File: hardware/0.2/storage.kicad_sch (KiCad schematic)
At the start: 8 parts, among them J1 Micro_SD_Card, U3 S27KS0641

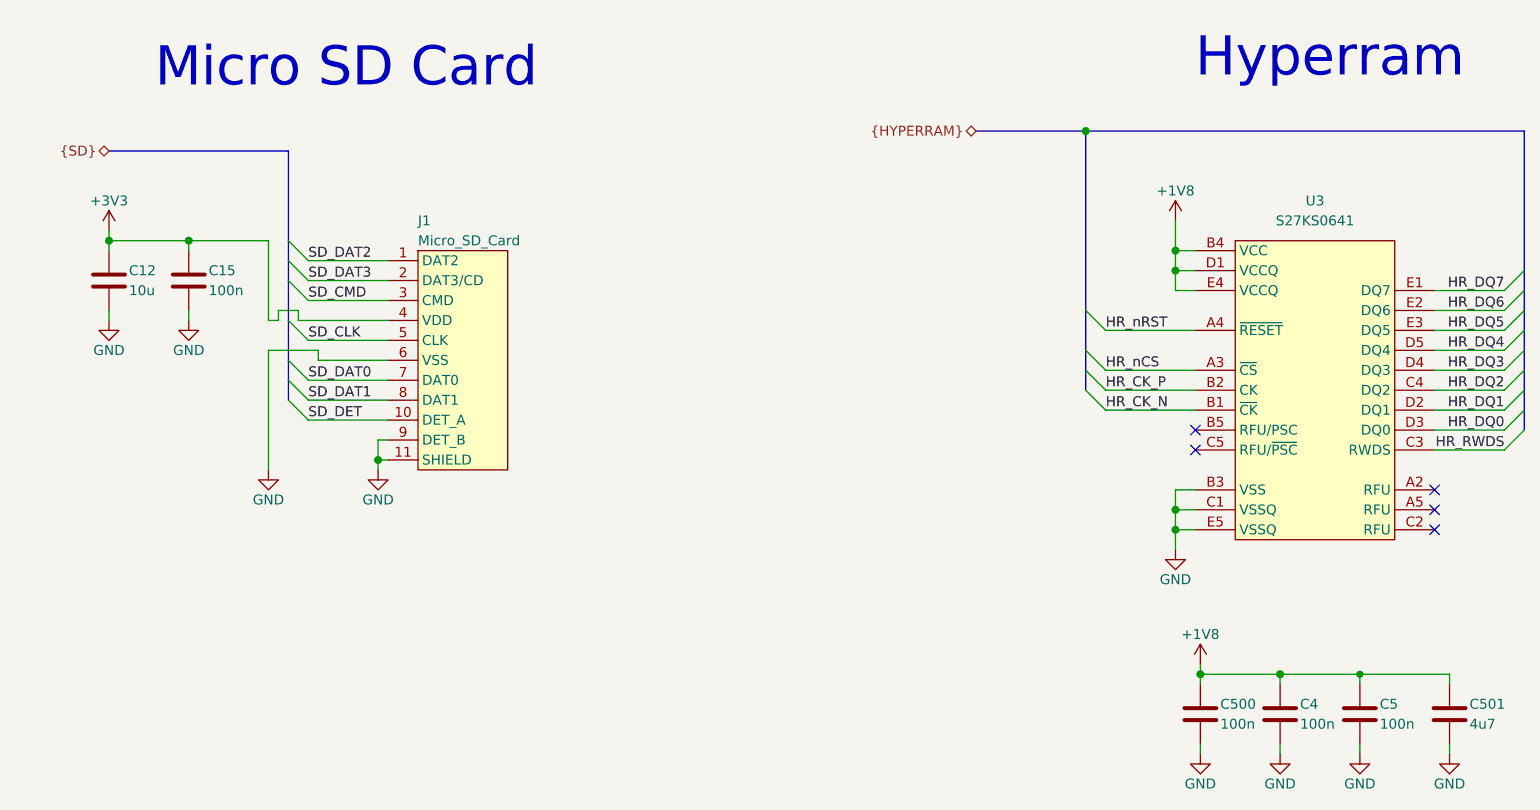
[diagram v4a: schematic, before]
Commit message: nightly version bump
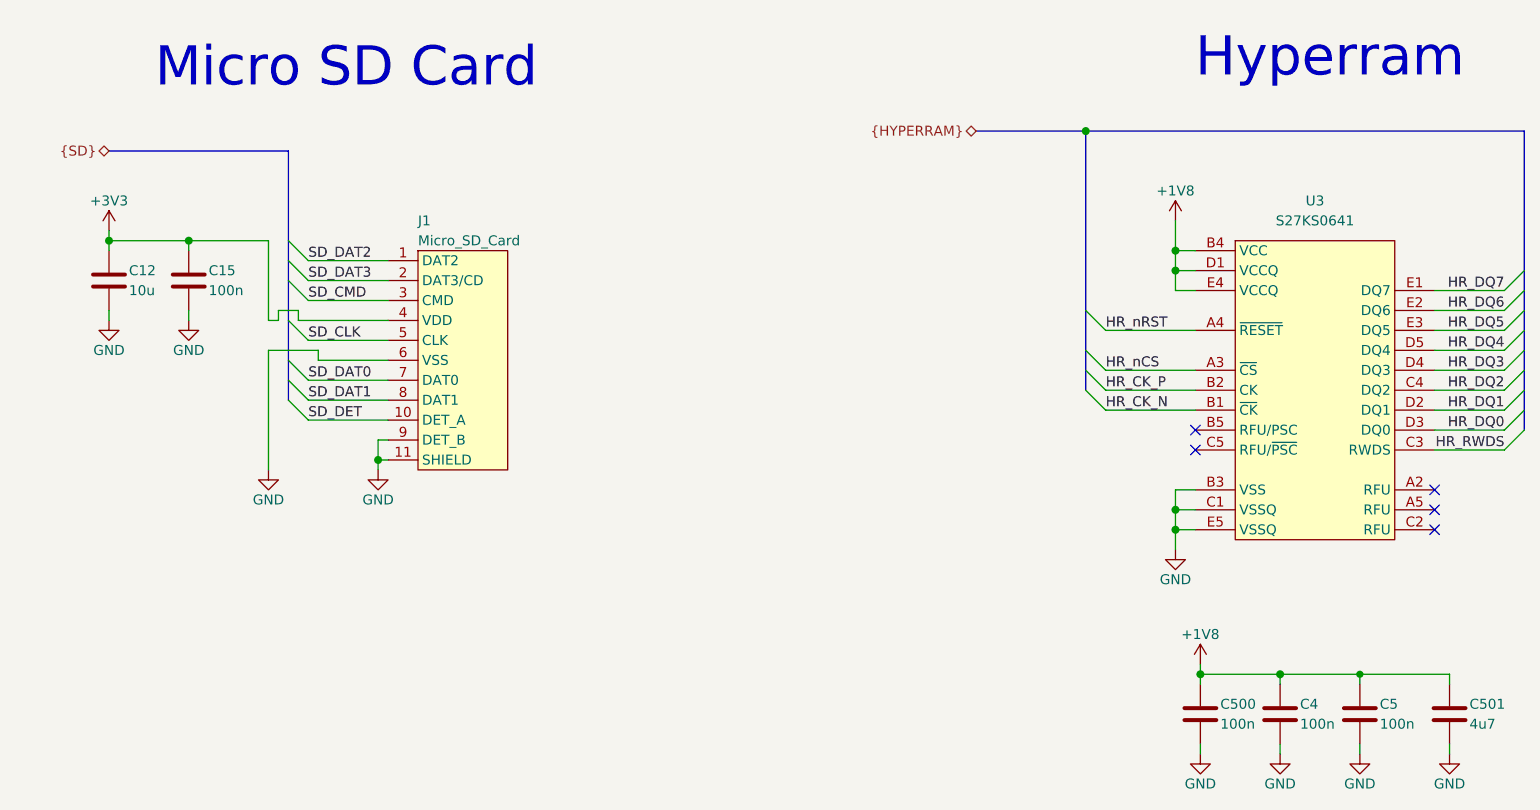
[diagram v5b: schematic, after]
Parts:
- C12: MPN2 CL10A106KP8NNNC -> (none)
- C15, C4, C5, C500: MPN2 CL05B104KO5NNNC -> (none)
- C501: MPN2 CL05A475KP5NRNC -> (none)
- U3: MPN2 IS66WVH8M8ALL-166B1LI -> (none)
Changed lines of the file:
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@@
-(kicad_sch (version 20210126) (generator eeschema)
+(kicad_sch (version 20210406) (generator eeschema)
   (paper "A4")
   (title_block
@@
     (stroke (width 0) (type solid) (color 0 0 0 0))
   )
-  (bus (pts (xy 82.55 73.66) (xy 82.55 62.23))
-    (stroke (width 0) (type solid) (color 0 0 0 0))
-  )
-  (bus (pts (xy 82.55 73.66) (xy 82.55 76.2))
-    (stroke (width 0) (type solid) (color 0 0 0 0))
-  )
-  (bus (pts (xy 82.55 76.2) (xy 82.55 78.74))
-    (stroke (width 0) (type solid) (color 0 0 0 0))
-  )
-  (bus (pts (xy 82.55 78.74) (xy 82.55 83.82))
-    (stroke (width 0) (type solid) (color 0 0 0 0))
-  )
-  (bus (pts (xy 82.55 83.82) (xy 82.55 88.9))
-    (stroke (width 0) (type solid) (color 0 0 0 0))
-  )
-  (bus (pts (xy 82.55 88.9) (xy 82.55 91.44))
-    (stroke (width 0) (type solid) (color 0 0 0 0))
-  )
-  (bus (pts (xy 82.55 91.44) (xy 82.55 93.98))
+  (bus (pts (xy 82.55 62.23) (xy 82.55 93.98))
     (stroke (width 0) (type solid) (color 0 0 0 0))
   )
@@
     (stroke (width 0) (type solid) (color 0 0 0 0))
   )
-  (bus (pts (xy 184.15 59.69) (xy 184.15 82.55))
+  (bus (pts (xy 184.15 59.69) (xy 184.15 92.71))
     (stroke (width 0) (type solid) (color 0 0 0 0))
   )
@@
     (stroke (width 0) (type solid) (color 0 0 0 0))
   )
-  (bus (pts (xy 184.15 82.55) (xy 184.15 87.63))
-    (stroke (width 0) (type solid) (color 0 0 0 0))
-  )
-  (bus (pts (xy 184.15 87.63) (xy 184.15 90.17))
-    (stroke (width 0) (type solid) (color 0 0 0 0))
-  )
-  (bus (pts (xy 184.15 90.17) (xy 184.15 92.71))
-    (stroke (width 0) (type solid) (color 0 0 0 0))
-  )
-  (bus (pts (xy 240.03 59.69) (xy 240.03 77.47))
-    (stroke (width 0) (type solid) (color 0 0 0 0))
-  )
-  (bus (pts (xy 240.03 77.47) (xy 240.03 80.01))
-    (stroke (width 0) (type solid) (color 0 0 0 0))
-  )
-  (bus (pts (xy 240.03 80.01) (xy 240.03 82.55))
-    (stroke (width 0) (type solid) (color 0 0 0 0))
-  )
-  (bus (pts (xy 240.03 82.55) (xy 240.03 85.09))
-    (stroke (width 0) (type solid) (color 0 0 0 0))
-  )
-  (bus (pts (xy 240.03 85.09) (xy 240.03 87.63))
-    (stroke (width 0) (type solid) (color 0 0 0 0))
-  )
-  (bus (pts (xy 240.03 87.63) (xy 240.03 90.17))
-    (stroke (width 0) (type solid) (color 0 0 0 0))
-  )
-  (bus (pts (xy 240.03 90.17) (xy 240.03 92.71))
-    (stroke (width 0) (type solid) (color 0 0 0 0))
-  )
-  (bus (pts (xy 240.03 92.71) (xy 240.03 95.25))
-    (stroke (width 0) (type solid) (color 0 0 0 0))
-  )
-  (bus (pts (xy 240.03 95.25) (xy 240.03 97.79))
+  (bus (pts (xy 240.03 59.69) (xy 240.03 97.79))
     (stroke (width 0) (type solid) (color 0 0 0 0))
   )
@@
       (effects (font (size 1.27 1.27)) hide)
     )
-    (property "MPN2" "CL10A106KP8NNNC" (id 4) (at 59.69 78.74 0)
-      (effects (font (size 1.27 1.27)) hide)
-    )
-    (property "Manufacturer2" "Samsung Electro-Mechanics" (id 5) (at 59.69 78.74 0)
+    (property "Manufacturer2" "Samsung Electro-Mechanics" (id 7) (at 59.69 78.74 0)
       (effects (font (size 1.27 1.27)) hide)
     )
@@
       (effects (font (size 1.27 1.27)) hide)
     )
-    (property "MPN2" "CL05B104KO5NNNC" (id 4) (at 69.85 78.74 0)
-      (effects (font (size 1.27 1.27)) hide)
-    )
-    (property "Manufacturer2" "Samsung Electro-Mechanics" (id 5) (at 69.85 78.74 0)
+    (property "Manufacturer2" "Samsung Electro-Mechanics" (id 7) (at 69.85 78.74 0)
       (effects (font (size 1.27 1.27)) hide)
     )
@@
       (effects (font (size 1.27 1.27)) hide)
     )
-    (property "MPN2" "CL05B104KO5NNNC" (id 4) (at 198.755 133.985 0)
-      (effects (font (size 1.27 1.27)) hide)
-    )
-    (property "Manufacturer2" "Samsung Electro-Mechanics" (id 5) (at 198.755 133.985 0)
+    (property "Manufacturer2" "Samsung Electro-Mechanics" (id 7) (at 198.755 133.985 0)
       (effects (font (size 1.27 1.27)) hide)
     )
@@
       (effects (font (size 1.27 1.27)) hide)
     )
-    (property "MPN2" "CL05B104KO5NNNC" (id 4) (at 208.915 133.985 0)
-      (effects (font (size 1.27 1.27)) hide)
-    )
-    (property "Manufacturer2" "Samsung Electro-Mechanics" (id 5) (at 208.915 133.985 0)
+    (property "Manufacturer2" "Samsung Electro-Mechanics" (id 7) (at 208.915 133.985 0)
       (effects (font (size 1.27 1.27)) hide)
     )
@@
       (effects (font (size 1.27 1.27)) hide)
     )
-    (property "MPN2" "CL05B104KO5NNNC" (id 4) (at 219.075 133.985 0)
-      (effects (font (size 1.27 1.27)) hide)
-    )
-    (property "Manufacturer2" "Samsung Electro-Mechanics" (id 5) (at 219.075 133.985 0)
+    (property "Manufacturer2" "Samsung Electro-Mechanics" (id 7) (at 219.075 133.985 0)
       (effects (font (size 1.27 1.27)) hide)
     )
@@
       (effects (font (size 1.27 1.27)) hide)
     )
-    (property "MPN2" "CL05A475KP5NRNC" (id 4) (at 230.505 133.985 0)
-      (effects (font (size 1.27 1.27)) hide)
-    )
-    (property "Manufacturer2" "Samsung Electro-Mechanics" (id 5) (at 230.505 133.985 0)
+    (property "Manufacturer2" "Samsung Electro-Mechanics" (id 7) (at 230.505 133.985 0)
       (effects (font (size 1.27 1.27)) hide)
     )
@@
       (effects (font (size 1.27 1.27)) hide)
     )
-    (property "LCSC" "C585350" (id 4) (at 104.14 87.63 0)
+    (property "LCSC" "C585350" (id 6) (at 104.14 87.63 0)
       (effects (font (size 1.27 1.27)) hide)
     )
@@
       (effects (font (size 1.27 1.27)) hide)
     )
-    (property "MPN2" "IS66WVH8M8ALL-166B1LI" (id 4) (at 213.36 92.71 0)
-      (effects (font (size 1.27 1.27)) hide)
-    )
-    (property "Manufacturer2" "ISSI" (id 5) (at 213.36 92.71 0)
-      (effects (font (size 1.27 1.27)) hide)
-    )
+    (property "Manufacturer2" "ISSI" (id 6) (at 213.36 92.71 0)
+      (effects (font (size 1.27 1.27)) hide)
+    )
